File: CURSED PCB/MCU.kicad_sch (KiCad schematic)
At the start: 22 parts, among them U1 STM32G431KBT6, U3 MIC94090YC6, Y1 24MHz crystal

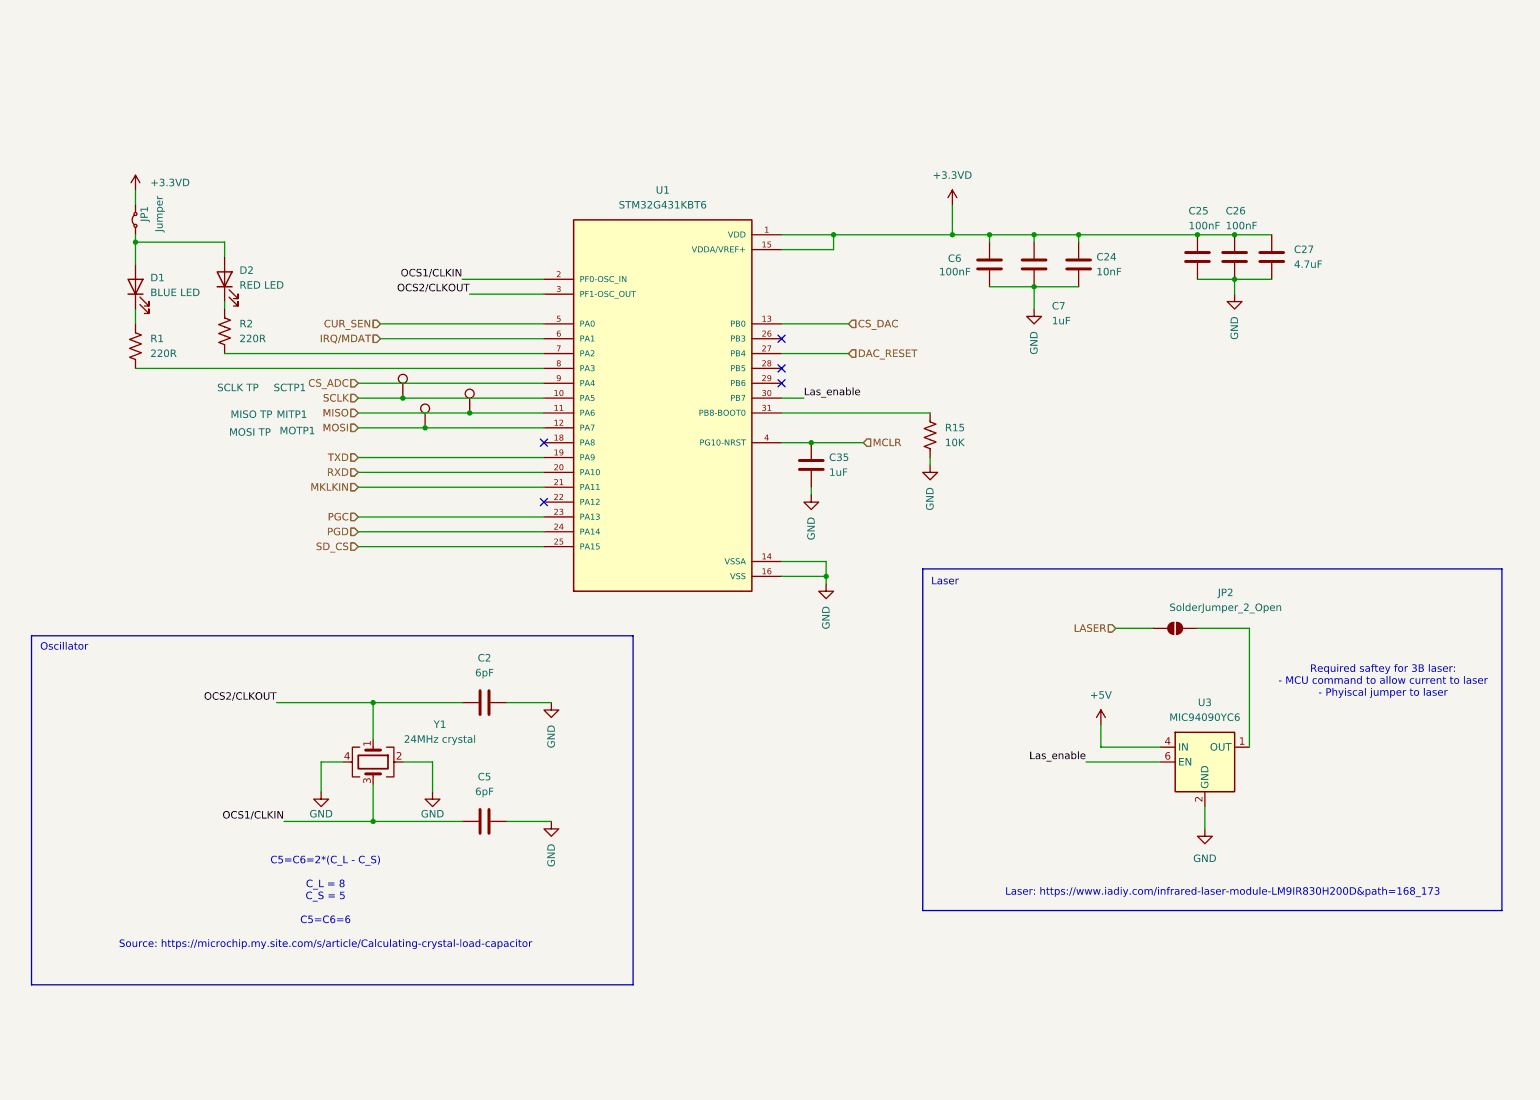
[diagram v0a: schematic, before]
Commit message: a
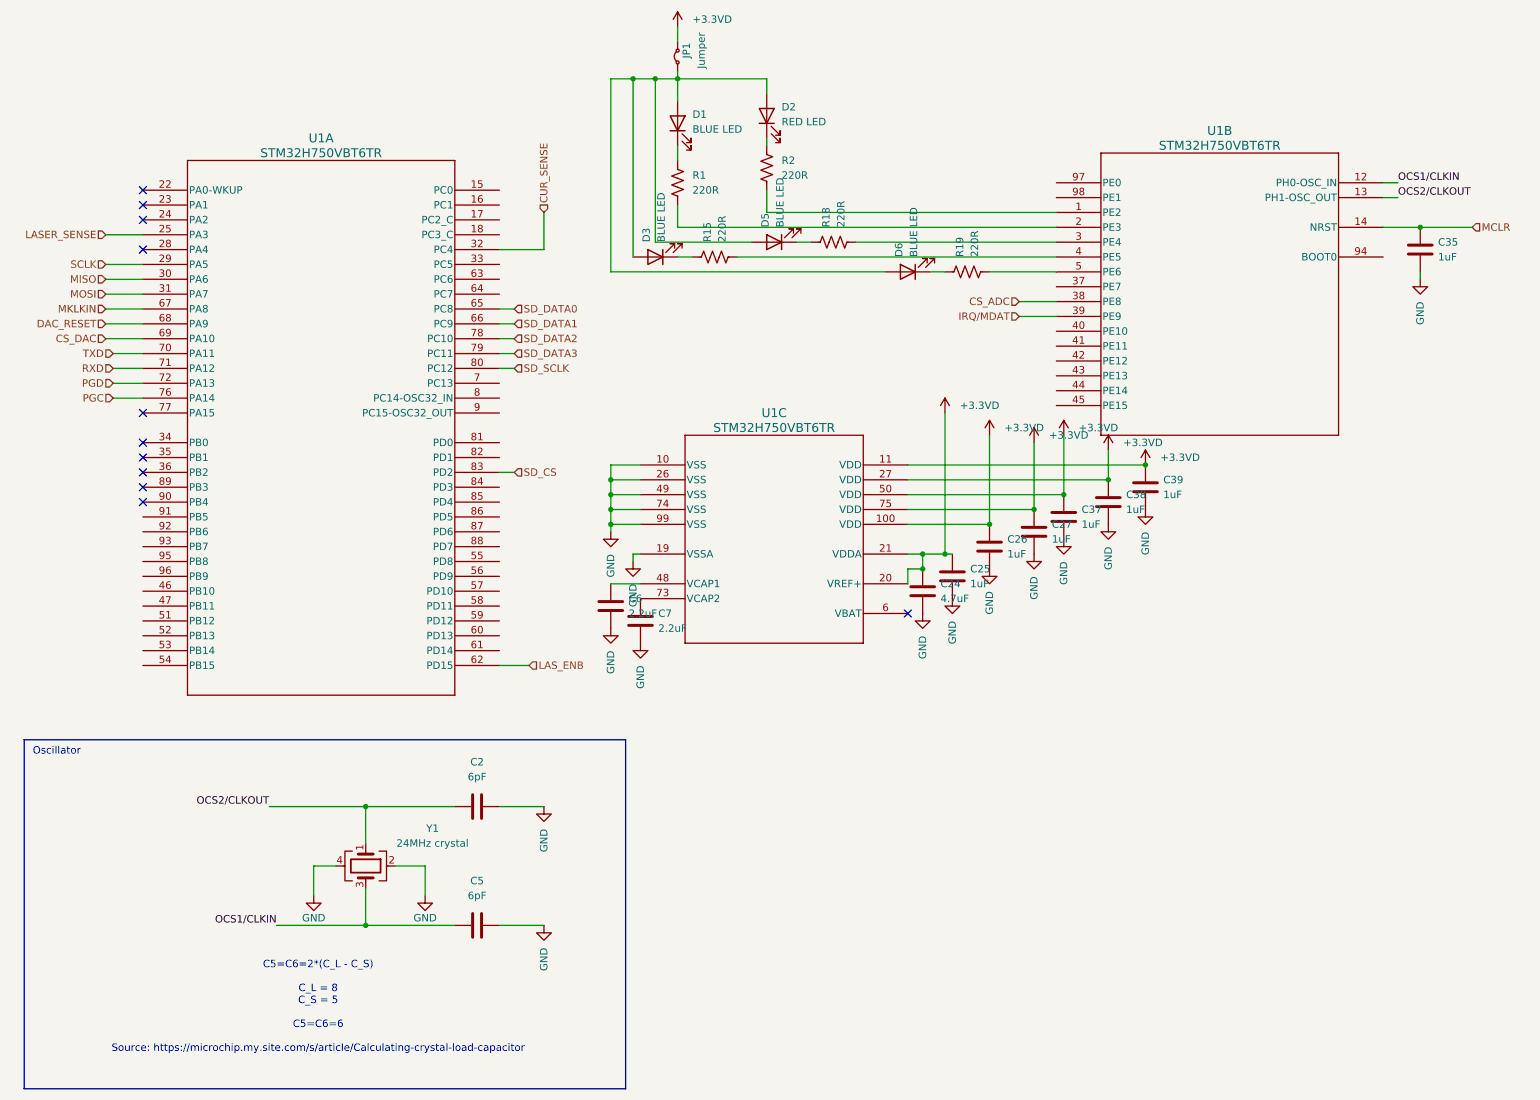
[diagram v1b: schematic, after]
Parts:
- removed JP2: SolderJumper_2_Open, Jumper:SolderJumper-2_P1.3mm_Open_Pad1.0x1.5mm, symbol Jumper:SolderJumper_2_Open
- removed MITP1: MISO TP, TestPoint:TestPoint_Pad_1.5x1.5mm, symbol Connector:TestPoint
- removed MOTP1: MOSI TP, TestPoint:TestPoint_Pad_1.5x1.5mm, symbol Connector:TestPoint
- removed SCTP1: SCLK TP, TestPoint:TestPoint_Pad_1.5x1.5mm, symbol Connector:TestPoint
- removed U1: STM32G431KBT6, STM32G431KBT6:QFP80P900X900X160-32N, symbol STM32G431KBT6:STM32G431KBT6
- removed U3: MIC94090YC6, Package_TO_SOT_SMD:SOT-363_SC-70-6, symbol Power_Management:MIC94090YC6
- added C37, C38, C39: 1uF, Capacitor_SMD:C_0603_1608Metric_Pad1.08x0.95mm_HandSolder, symbol PCM_Capacitor_US_AKL:C_0201
- added D3, D5, D6: BLUE LED, LED_SMD:LED_1206_3216Metric_Pad1.42x1.75mm_HandSolder, symbol Device:LED
- added R18, R19: 220R, Resistor_SMD:R_0603_1608Metric_Pad0.98x0.95mm_HandSolder, symbol Device:R_US
- added U1: STM32H750VBT6TR, Package_QFP:LQFP-100_14x14mm_P0.5mm, symbol STM32H750VBT6TR:STM32H750VBT6TR
- C24: value 10nF -> 4.7uF
- C25, C26: value 100nF -> 1uF
- C27: value 4.7uF -> 1uF
- C6: value 100nF -> 2.2uF
- C7: value 1uF -> 2.2uF
- JP1: footprint Jumper:SolderJumper-2_P1.3mm_Bridged2Bar_Pad1.0x1.5mm -> Connector_PinHeader_2.54mm:PinHeader_1x02_P2.54mm_Vertical
- R15: value 10K -> 220R
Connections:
- net +3.3VD: now also C37.2, C38.2, C39.2, U1.100 (VDD), U1.11 (VDD), U1.20 (VREF+), U1.21 (VDDA), U1.27 (VDD), U1.50 (VDD), U1.75 (VDD); no longer C6.1, C7.2
- net CS_ADC: now also U1.38 (PE8)
- net CS_DAC: now also U1.69 (PA10)
- net DAC_RESET: now also U1.68 (PA9)
- net GND: now also C6.1, C37.1, C38.1, C39.1, U1.10 (VSS), U1.19 (VSSA), U1.26 (VSS), U1.49 (VSS), U1.74 (VSS), U1.99 (VSS); no longer C6.2, R15.2
- net IRQ/MDAT: now also U1.39 (PE9)
- net MCLR: now also U1.14 (NRST)
- net MISO: now also U1.30 (PA6)
- net MKLKIN: now also U1.67 (PA8)
- net MOSI: now also U1.31 (PA7)
- net OCS1/CLKIN: now also U1.12 (PH0-OSC_IN)
- net OCS2/CLKOUT: now also U1.13 (PH1-OSC_OUT)
- net PGC: now also U1.76 (PA14)
- net PGD: now also U1.72 (PA13)
- net RXD: now also U1.71 (PA12)
- net SCLK: now also U1.29 (PA5)
- net SD_CS: now also U1.83 (PD2)
- net TXD: now also U1.70 (PA11)
- net at D1.2 (A), D2.2 (A), JP1.1 (A): now also D3.2 (A), D5.2 (A), D6.2 (A)
- net at R15.1: now also D3.1 (K)
- net at R2.2: now also U1.1 (PE2)
- net at R1.2: now also U1.2 (PE3)
- new net: C7.2, U1.73 (VCAP2)
- new net: D6.1 (K), R19.1
- new net: R19.2, U1.5 (PE6)
- new net: D5.1 (K), R18.1
- new net: R18.2, U1.3 (PE4)
- new net: C6.2, U1.48 (VCAP1)
- new net: R15.2, U1.4 (PE5)
- new net CUR_SENSE: U1.32 (PC4)
- new net LASER_SENSE: U1.25 (PA3)
- new net LAS_ENB: U1.62 (PD15)
- new net SD_DATA0: U1.65 (PC8)
- new net SD_DATA1: U1.66 (PC9)
- new net SD_DATA2: U1.78 (PC10)
- new net SD_DATA3: U1.79 (PC11)
- new net SD_SCLK: U1.80 (PC12)
- no-connect marks 5 -> 11
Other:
- note removed: "Laser"
- note removed: "Laser: https://www.iadiy.com/infrared-laser-module-LM9IR830H200D&path=168_173"
- note removed: "Required saftey for 3B laser: - MCU command to allow current to laser - Phyiscal jumper to laser"
- moved on the sheet: C2, C35, C5, D1, D2, JP1, R2, Y1
